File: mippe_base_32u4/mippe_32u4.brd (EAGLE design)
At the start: 31 x 37 mm, 32 parts, among them J2 USB, J5 BURNIN, SW1 BTN-PTS810, U1 ATMEGA32U4-XUMU, U2 MIPPE, Y1 16MHz

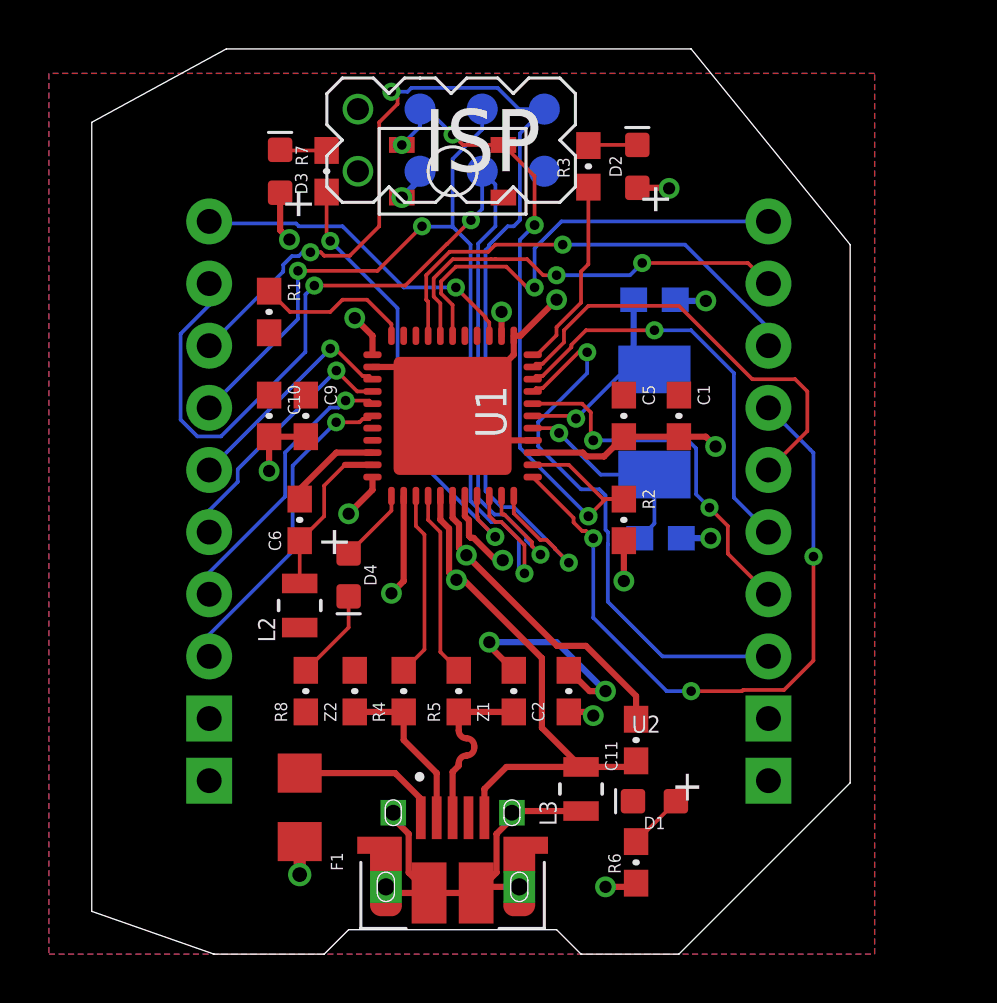
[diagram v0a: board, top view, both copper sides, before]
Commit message: Add files for jlc order
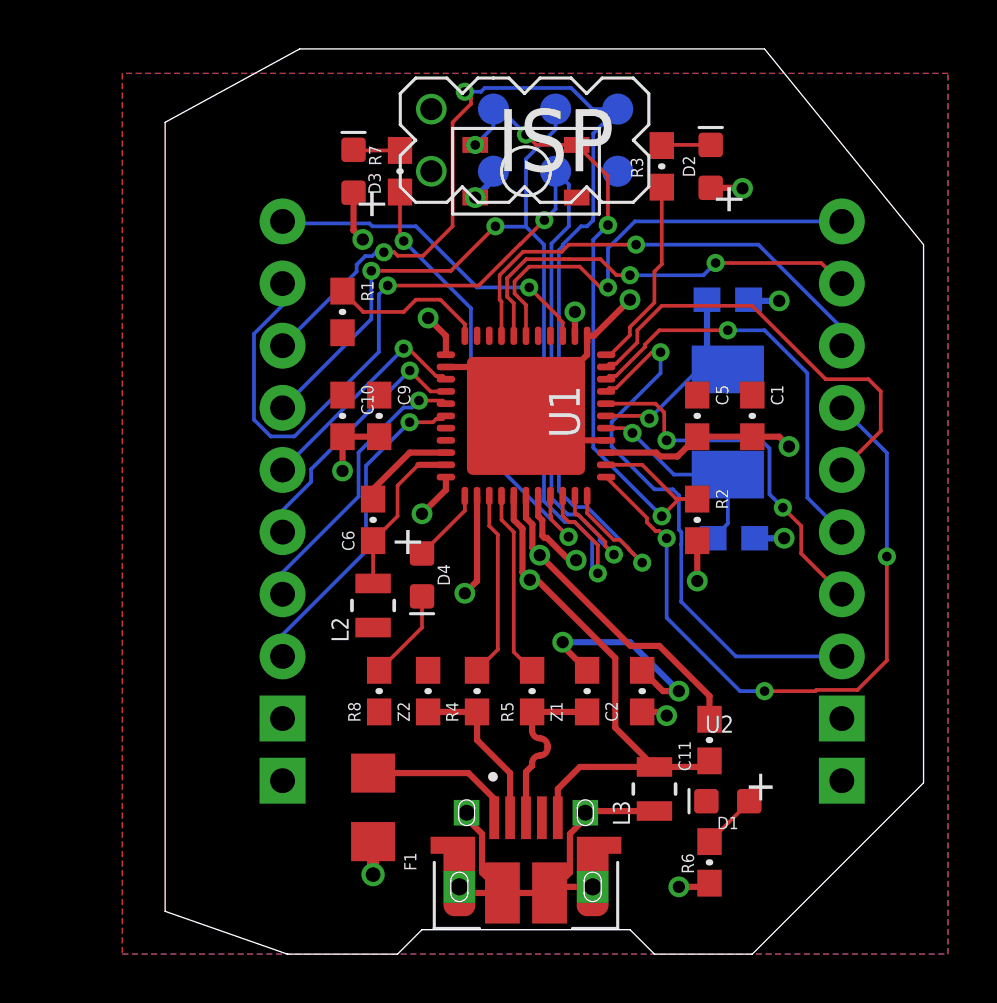
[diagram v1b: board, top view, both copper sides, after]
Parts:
- moved C1 3.00 mm to (24.0, 22.0)
- moved C10 3.00 mm to (7.25, 22.0)
- moved C11 3.00 mm to (22.2, 8.75)
- moved C2 3.00 mm to (19.5, 10.8)
- moved C3 3.00 mm to (23.0, 26.8)
- moved C4 3.00 mm to (23.2, 17.0)
- moved C5 3.00 mm to (21.8, 22.0)
- moved C6 3.00 mm to (8.50, 17.8)
- moved C9 3.00 mm to (8.75, 22.0)
- moved D1 3.00 mm to (23.0, 6.25)
- moved D2 3.00 mm to (22.3, 32.2)
- moved D3 3.00 mm to (7.70, 32.0)
- moved D4 3.00 mm to (10.5, 15.5)
- moved F1 3.00 mm to (8.50, 6.00)
- moved J2 3.00 mm to (14.8, 2.75)
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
